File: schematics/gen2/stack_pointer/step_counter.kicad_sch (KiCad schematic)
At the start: 16 parts, among them J1 Bus_PCI_Express_x16, U1 74LS00, U2 74LS193, U3 74LS193, U4 74LS193, U5 74LS193, U6 74LS245, U7 74LS245

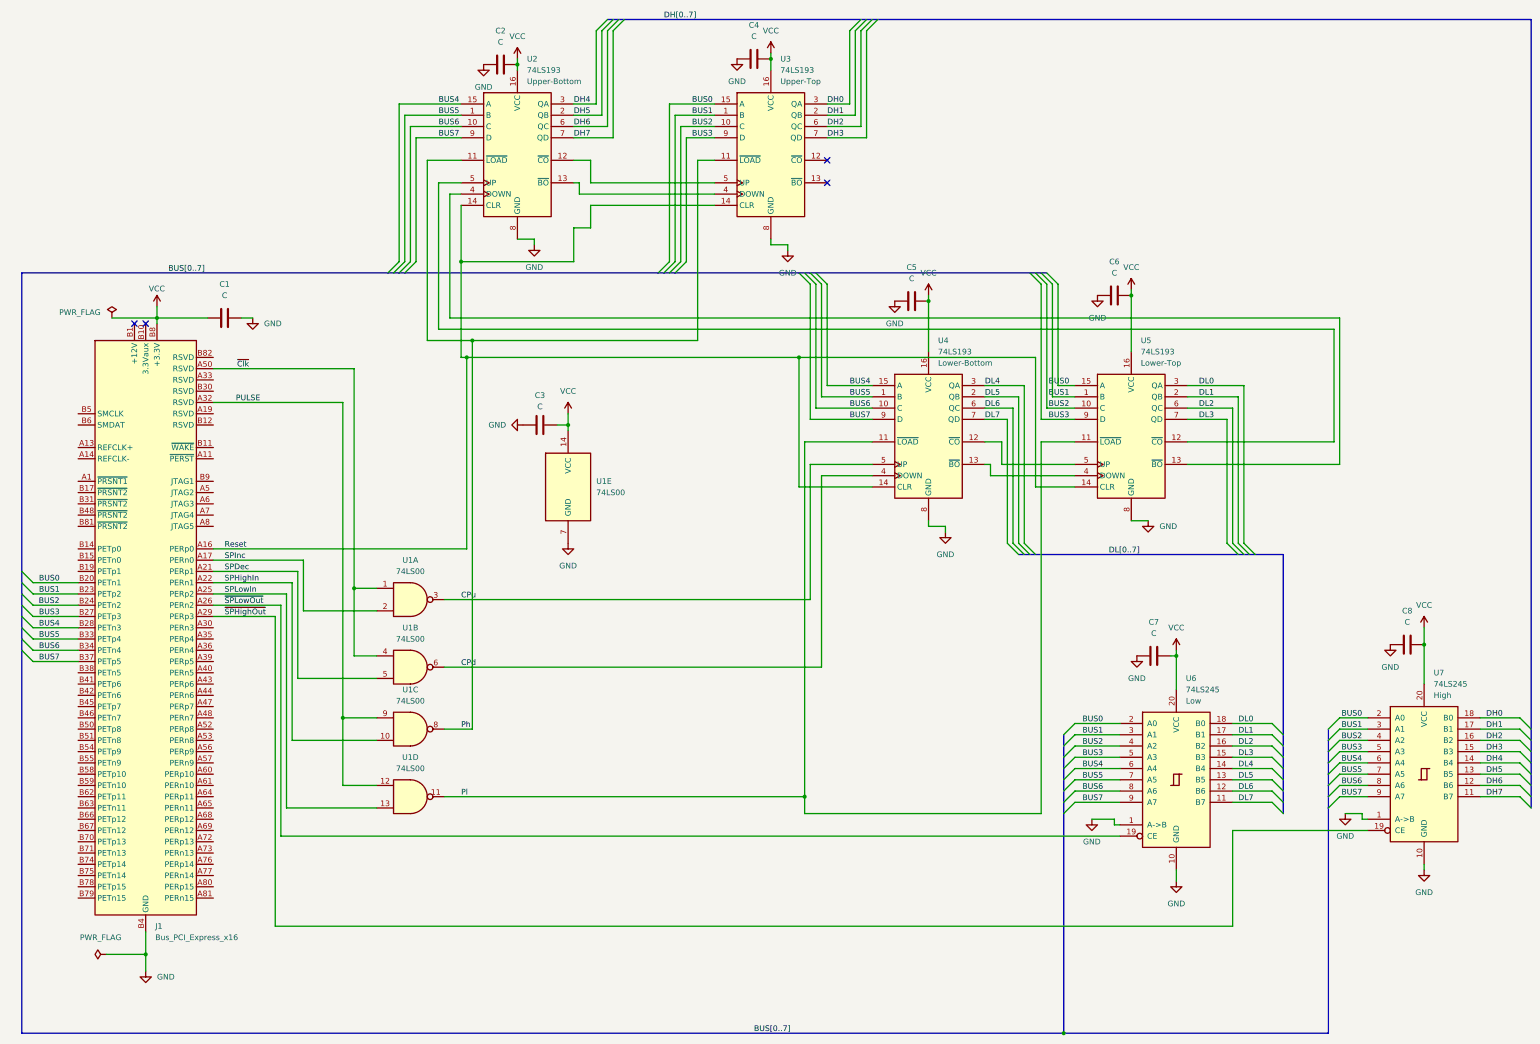
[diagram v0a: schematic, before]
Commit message: (feat) step_counter update.
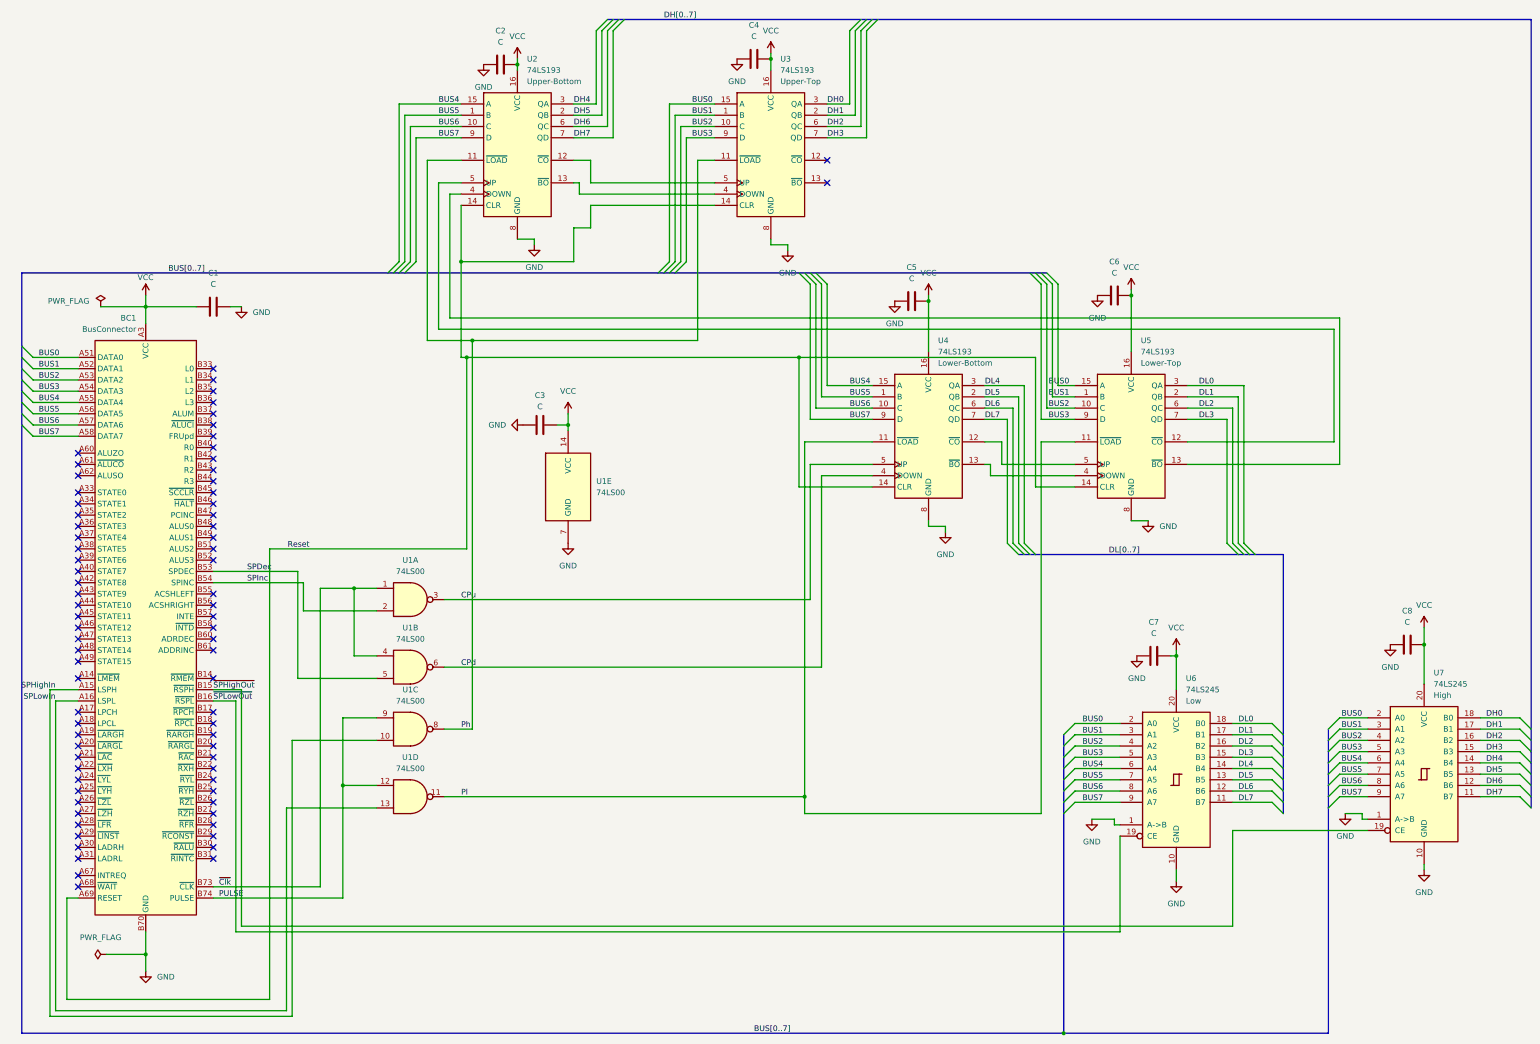
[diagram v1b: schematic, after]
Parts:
- removed J1: Bus_PCI_Express_x16, Connector_PCBEdge:BUS_PCIexpress_x16, symbol Connector:Bus_PCI_Express_x16
- added BC1: BusConnector, Connector_PCBEdge:BUS_PCIexpress_x16, symbol cpu816symbols:BusConnector
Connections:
- net BUS0: now also BC1.A51 (DATA0)
- net BUS1: now also BC1.A52 (DATA1)
- net BUS2: now also BC1.A53 (DATA2)
- net BUS3: now also BC1.A54 (DATA3)
- net BUS4: now also BC1.A55 (DATA4)
- net BUS5: now also BC1.A56 (DATA5)
- net BUS6: now also BC1.A57 (DATA6)
- net BUS7: now also BC1.A58 (DATA7)
- net GND: now also BC1.A12 (GND), BC1.A13 (GND), BC1.A23 (GND), BC1.A32 (GND), BC1.A41 (GND), BC1.A50 (GND), BC1.A59 (GND), BC1.A63 (GND), BC1.A64 (GND), BC1.A65 (GND), BC1.A66 (GND), BC1.A70 (GND), BC1.A71 (GND), BC1.A72 (GND), BC1.A73 (GND), BC1.A74 (GND), BC1.A75 (GND), BC1.A76 (GND), BC1.B12 (GND), BC1.B13 (GND), BC1.B23 (GND), BC1.B32 (GND), BC1.B41 (GND), BC1.B50 (GND), BC1.B59 (GND), BC1.B62 (GND), BC1.B63 (GND), BC1.B64 (GND), BC1.B65 (GND), BC1.B66 (GND), BC1.B67 (GND), BC1.B68 (GND), BC1.B69 (GND), BC1.B70 (GND), BC1.B71 (GND), BC1.B72 (GND), BC1.B75 (GND), BC1.B76 (GND)
- net PULSE: now also BC1.B74 (PULSE)
- net Reset: now also BC1.A69 (RESET)
- net SPDec: now also BC1.B53 (SPDEC)
- net SPHighIn: now also BC1.A15 (LSPH)
- net SPInc: now also BC1.B54 (SPINC)
- net SPLowIn: now also BC1.A16 (LSPL)
- net VCC: now also BC1.A1 (VCC), BC1.A2 (VCC), BC1.A3 (VCC), BC1.A4 (VCC), BC1.A5 (VCC), BC1.B1 (VCC), BC1.B2 (VCC), BC1.B3 (VCC), BC1.B4 (VCC), BC1.B5 (VCC)
- net ~{Clk}: now also BC1.B73 (~{CLK})
- net ~{SPHighOut}: now also BC1.B15 (~{RSPH})
- net ~{SPLowOut}: now also BC1.B16 (~{RSPL})
- no-connect marks 4 -> 77
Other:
- moved on the sheet: C1
